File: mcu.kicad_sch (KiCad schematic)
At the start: 5 parts, among them U1 MIMXRT1052CVJ5B

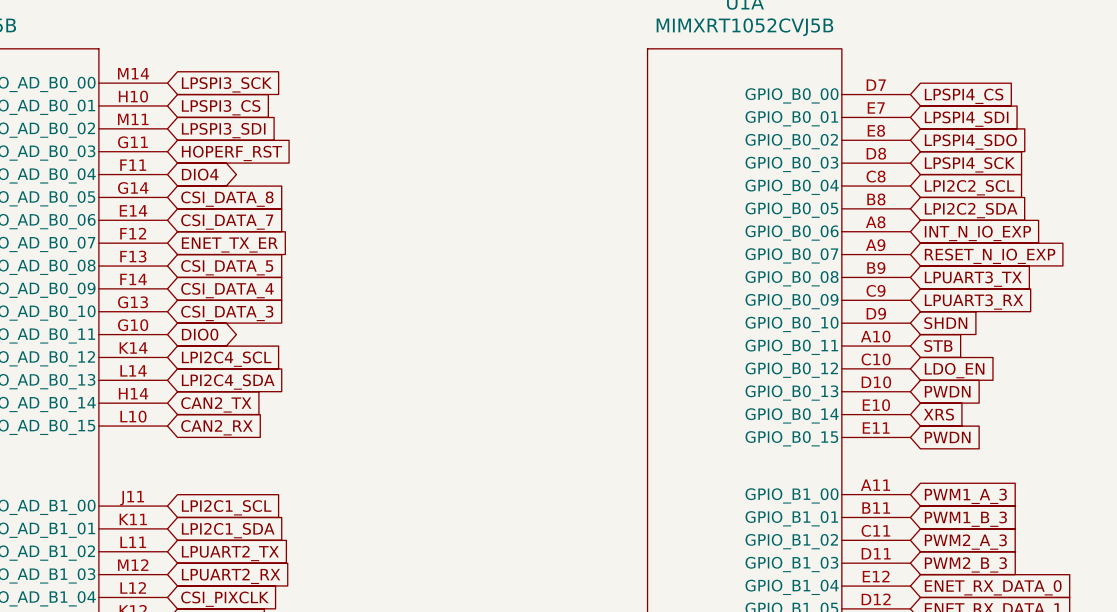
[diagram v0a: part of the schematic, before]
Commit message: save before sdram redesign
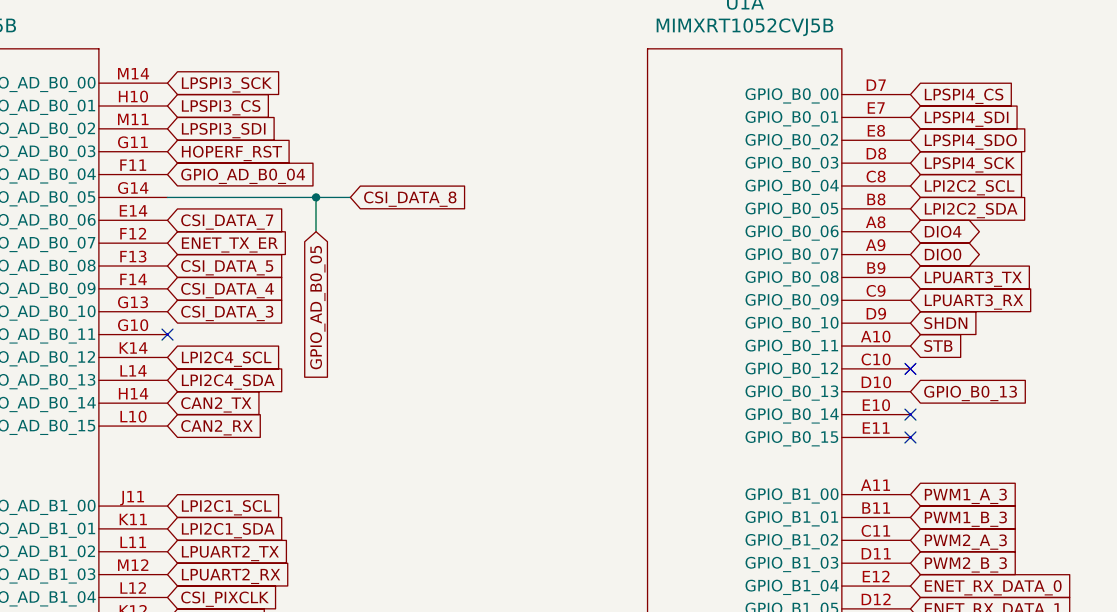
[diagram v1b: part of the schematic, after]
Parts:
- C58, C59, C60, C61: footprint Capacitor_SMD:C_0402_1005Metric -> Capacitor_SMD:C_0201_0603Metric
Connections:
- net INT_N_IO_EXP is gone; now on net DIO4: U1.A8 (GPIO_B0_06)
- net RESET_N_IO_EXP is gone; now on net DIO0: U1.A9 (GPIO_B0_07)
- net DIO0: no longer U1.G10 (GPIO_AD_B0_11)
- net DIO4: no longer U1.F11 (GPIO_AD_B0_04)
- net LDO_EN: no longer names the net of U1.C10 (GPIO_B0_12)
- net PWDN: no longer names the net of U1.E11 (GPIO_B0_15)
- net PWDN: no longer U1.D10 (GPIO_B0_13)
- net XRS: no longer names the net of U1.E10 (GPIO_B0_14)
- new net GPIO_AD_B0_04: U1.F11 (GPIO_AD_B0_04)
- new net GPIO_B0_13: U1.D10 (GPIO_B0_13)
- no-connect marks 0 -> 4
